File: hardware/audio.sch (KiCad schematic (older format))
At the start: 25 parts, among them U4 FM8002A, U5 TM8211, U6 FM8002A

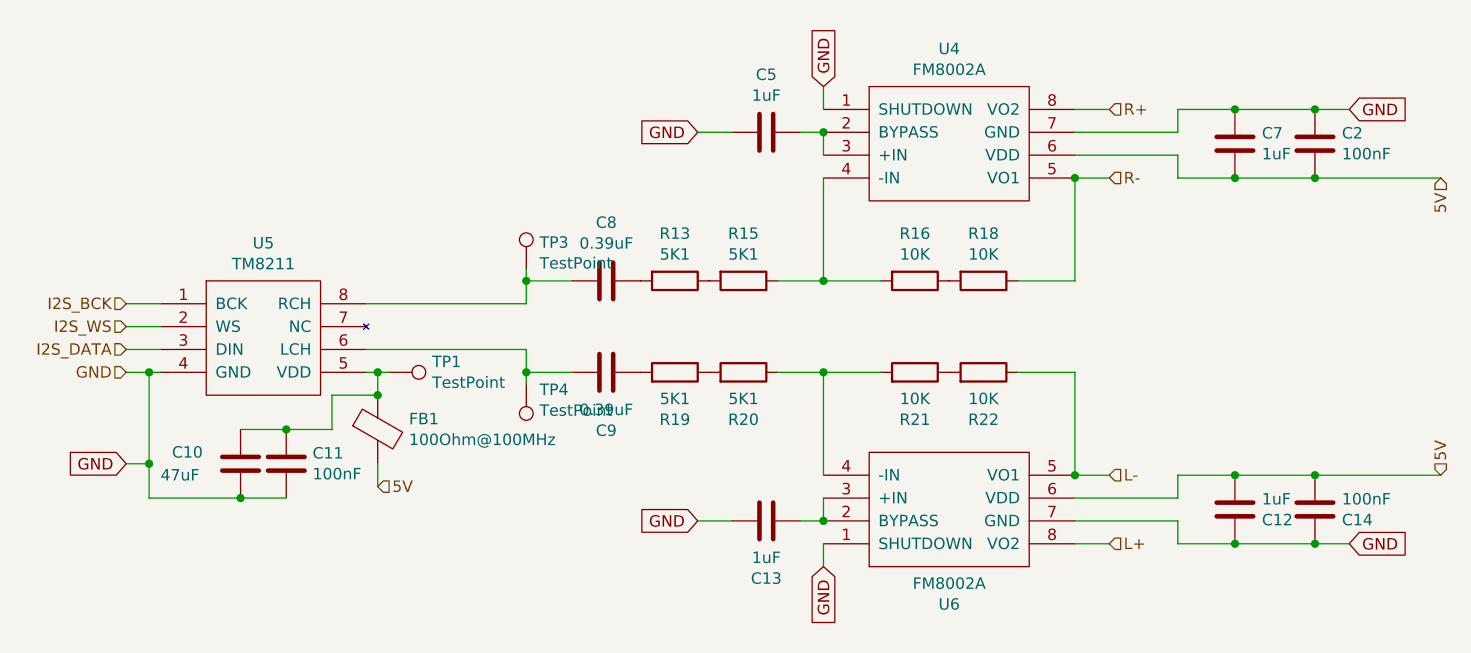
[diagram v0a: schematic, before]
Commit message: Production data rev4
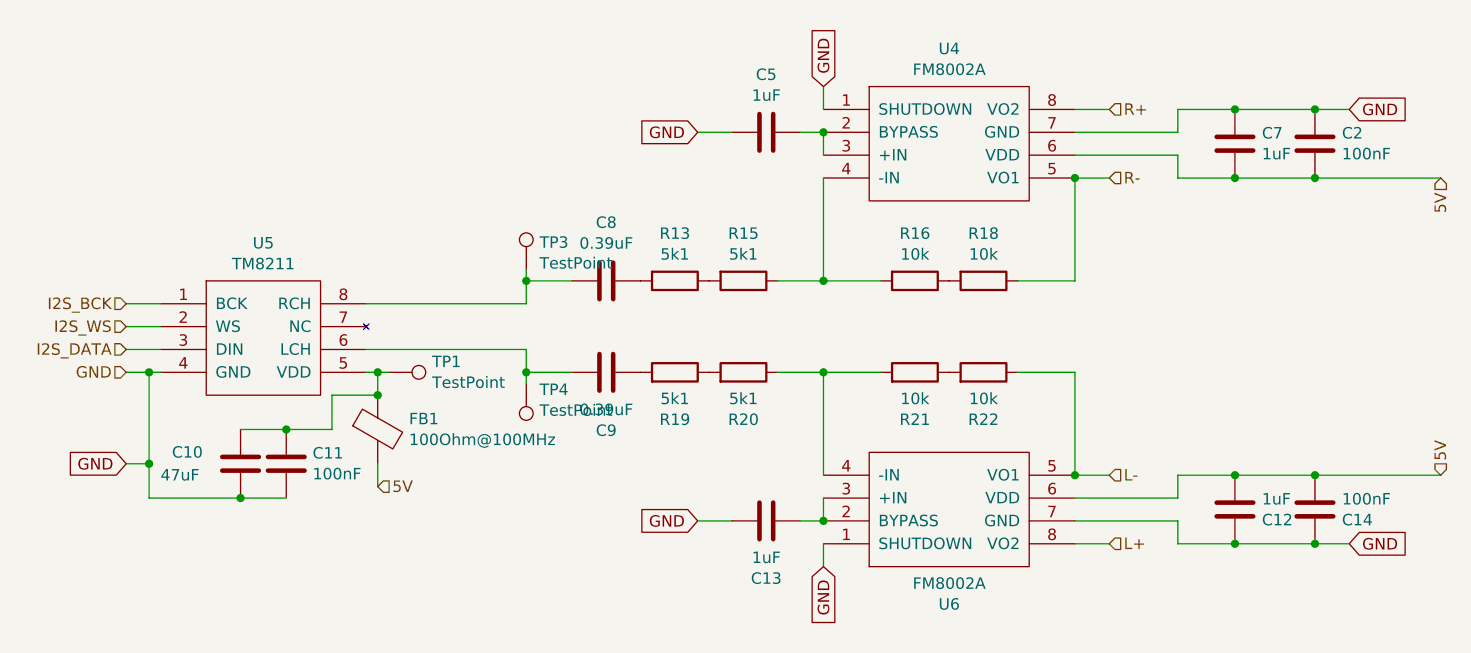
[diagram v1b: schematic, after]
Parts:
- R13, R15, R19, R20: value 5K1 -> 5k1
- R16, R18, R21, R22: value 10K -> 10k
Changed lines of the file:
@@
 P 5050 3050
 F 0 "R18" V 4843 3050 50  0000 C CNN
-F 1 "10K" V 4934 3050 50  0000 C CNN
+F 1 "10k" V 4934 3050 50  0000 C CNN
 F 2 "Resistor_SMD:R_0603_1608Metric" V 4980 3050 50  0001 C CNN
 F 3 "~" H 5050 3050 50  0001 C CNN
@@
 P 4750 3050
 F 0 "R16" V 4543 3050 50  0000 C CNN
-F 1 "10K" V 4634 3050 50  0000 C CNN
+F 1 "10k" V 4634 3050 50  0000 C CNN
 F 2 "Resistor_SMD:R_0603_1608Metric" V 4680 3050 50  0001 C CNN
 F 3 "~" H 4750 3050 50  0001 C CNN
@@
 P 4000 3050
 F 0 "R15" V 3793 3050 50  0000 C CNN
-F 1 "5K1" V 3884 3050 50  0000 C CNN
+F 1 "5k1" V 3884 3050 50  0000 C CNN
 F 2 "Resistor_SMD:R_0603_1608Metric" V 3930 3050 50  0001 C CNN
 F 3 "~" H 4000 3050 50  0001 C CNN
@@
 P 3700 3050
 F 0 "R13" V 3493 3050 50  0000 C CNN
-F 1 "5K1" V 3584 3050 50  0000 C CNN
+F 1 "5k1" V 3584 3050 50  0000 C CNN
 F 2 "Resistor_SMD:R_0603_1608Metric" V 3630 3050 50  0001 C CNN
 F 3 "~" H 3700 3050 50  0001 C CNN
@@
 P 5050 3450
 F 0 "R22" V 4843 3450 50  0000 C CNN
-F 1 "10K" V 4934 3450 50  0000 C CNN
+F 1 "10k" V 4934 3450 50  0000 C CNN
 F 2 "Resistor_SMD:R_0603_1608Metric" V 4980 3450 50  0001 C CNN
 F 3 "~" H 5050 3450 50  0001 C CNN
@@
 P 4750 3450
 F 0 "R21" V 4543 3450 50  0000 C CNN
-F 1 "10K" V 4634 3450 50  0000 C CNN
+F 1 "10k" V 4634 3450 50  0000 C CNN
 F 2 "Resistor_SMD:R_0603_1608Metric" V 4680 3450 50  0001 C CNN
 F 3 "~" H 4750 3450 50  0001 C CNN
@@
 P 4000 3450
 F 0 "R20" V 3793 3450 50  0000 C CNN
-F 1 "5K1" V 3884 3450 50  0000 C CNN
+F 1 "5k1" V 3884 3450 50  0000 C CNN
 F 2 "Resistor_SMD:R_0603_1608Metric" V 3930 3450 50  0001 C CNN
 F 3 "~" H 4000 3450 50  0001 C CNN
@@
 P 3700 3450
 F 0 "R19" V 3493 3450 50  0000 C CNN
-F 1 "5K1" V 3584 3450 50  0000 C CNN
+F 1 "5k1" V 3584 3450 50  0000 C CNN
 F 2 "Resistor_SMD:R_0603_1608Metric" V 3630 3450 50  0001 C CNN
 F 3 "~" H 3700 3450 50  0001 C CNN

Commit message: Updated production files: - vias in 8-pin female header - fixed some text elements - added testpoint for FLASH
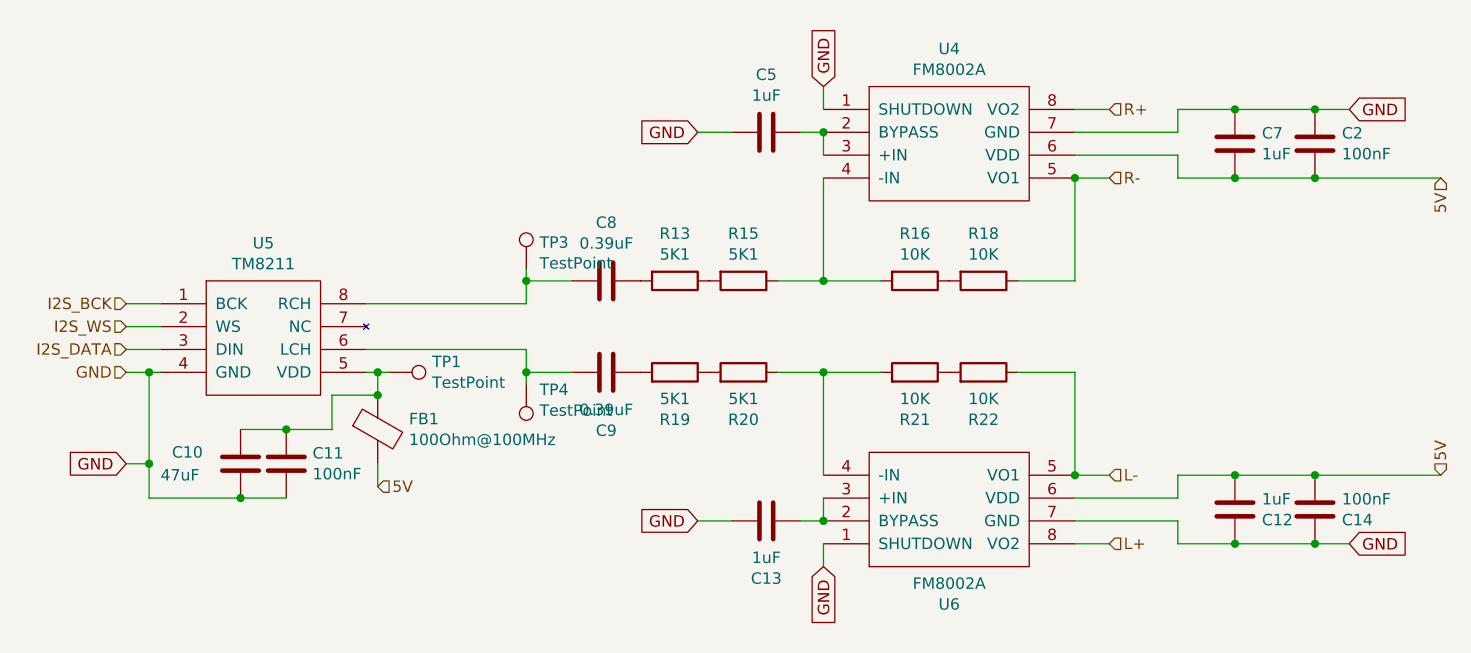
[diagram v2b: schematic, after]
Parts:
- R13, R15, R19, R20: value 5k1 -> 5K1
- R16, R18, R21, R22: value 10k -> 10K
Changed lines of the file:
@@
 P 5050 3050
 F 0 "R18" V 4843 3050 50  0000 C CNN
-F 1 "10k" V 4934 3050 50  0000 C CNN
+F 1 "10K" V 4934 3050 50  0000 C CNN
 F 2 "Resistor_SMD:R_0603_1608Metric" V 4980 3050 50  0001 C CNN
 F 3 "~" H 5050 3050 50  0001 C CNN
@@
 P 4750 3050
 F 0 "R16" V 4543 3050 50  0000 C CNN
-F 1 "10k" V 4634 3050 50  0000 C CNN
+F 1 "10K" V 4634 3050 50  0000 C CNN
 F 2 "Resistor_SMD:R_0603_1608Metric" V 4680 3050 50  0001 C CNN
 F 3 "~" H 4750 3050 50  0001 C CNN
@@
 P 4000 3050
 F 0 "R15" V 3793 3050 50  0000 C CNN
-F 1 "5k1" V 3884 3050 50  0000 C CNN
+F 1 "5K1" V 3884 3050 50  0000 C CNN
 F 2 "Resistor_SMD:R_0603_1608Metric" V 3930 3050 50  0001 C CNN
 F 3 "~" H 4000 3050 50  0001 C CNN
@@
 P 3700 3050
 F 0 "R13" V 3493 3050 50  0000 C CNN
-F 1 "5k1" V 3584 3050 50  0000 C CNN
+F 1 "5K1" V 3584 3050 50  0000 C CNN
 F 2 "Resistor_SMD:R_0603_1608Metric" V 3630 3050 50  0001 C CNN
 F 3 "~" H 3700 3050 50  0001 C CNN
@@
 P 5050 3450
 F 0 "R22" V 4843 3450 50  0000 C CNN
-F 1 "10k" V 4934 3450 50  0000 C CNN
+F 1 "10K" V 4934 3450 50  0000 C CNN
 F 2 "Resistor_SMD:R_0603_1608Metric" V 4980 3450 50  0001 C CNN
 F 3 "~" H 5050 3450 50  0001 C CNN
@@
 P 4750 3450
 F 0 "R21" V 4543 3450 50  0000 C CNN
-F 1 "10k" V 4634 3450 50  0000 C CNN
+F 1 "10K" V 4634 3450 50  0000 C CNN
 F 2 "Resistor_SMD:R_0603_1608Metric" V 4680 3450 50  0001 C CNN
 F 3 "~" H 4750 3450 50  0001 C CNN
@@
 P 4000 3450
 F 0 "R20" V 3793 3450 50  0000 C CNN
-F 1 "5k1" V 3884 3450 50  0000 C CNN
+F 1 "5K1" V 3884 3450 50  0000 C CNN
 F 2 "Resistor_SMD:R_0603_1608Metric" V 3930 3450 50  0001 C CNN
 F 3 "~" H 4000 3450 50  0001 C CNN
@@
 P 3700 3450
 F 0 "R19" V 3493 3450 50  0000 C CNN
-F 1 "5k1" V 3584 3450 50  0000 C CNN
+F 1 "5K1" V 3584 3450 50  0000 C CNN
 F 2 "Resistor_SMD:R_0603_1608Metric" V 3630 3450 50  0001 C CNN
 F 3 "~" H 3700 3450 50  0001 C CNN
